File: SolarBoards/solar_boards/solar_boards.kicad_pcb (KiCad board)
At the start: 2 copper layers, 51.8 x 47 mm, 5 parts, among them J1 M55-6001242R

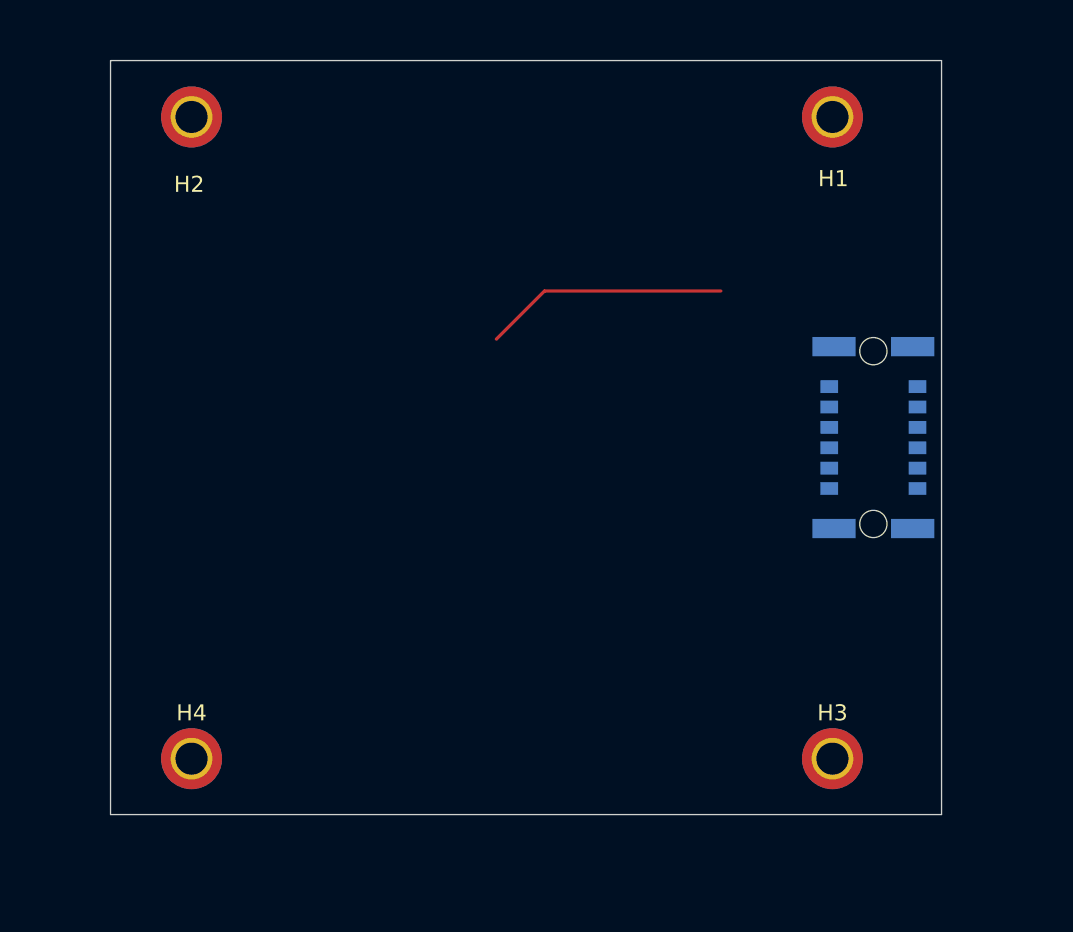
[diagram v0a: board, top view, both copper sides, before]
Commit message: Solar Board Schematic and Routing
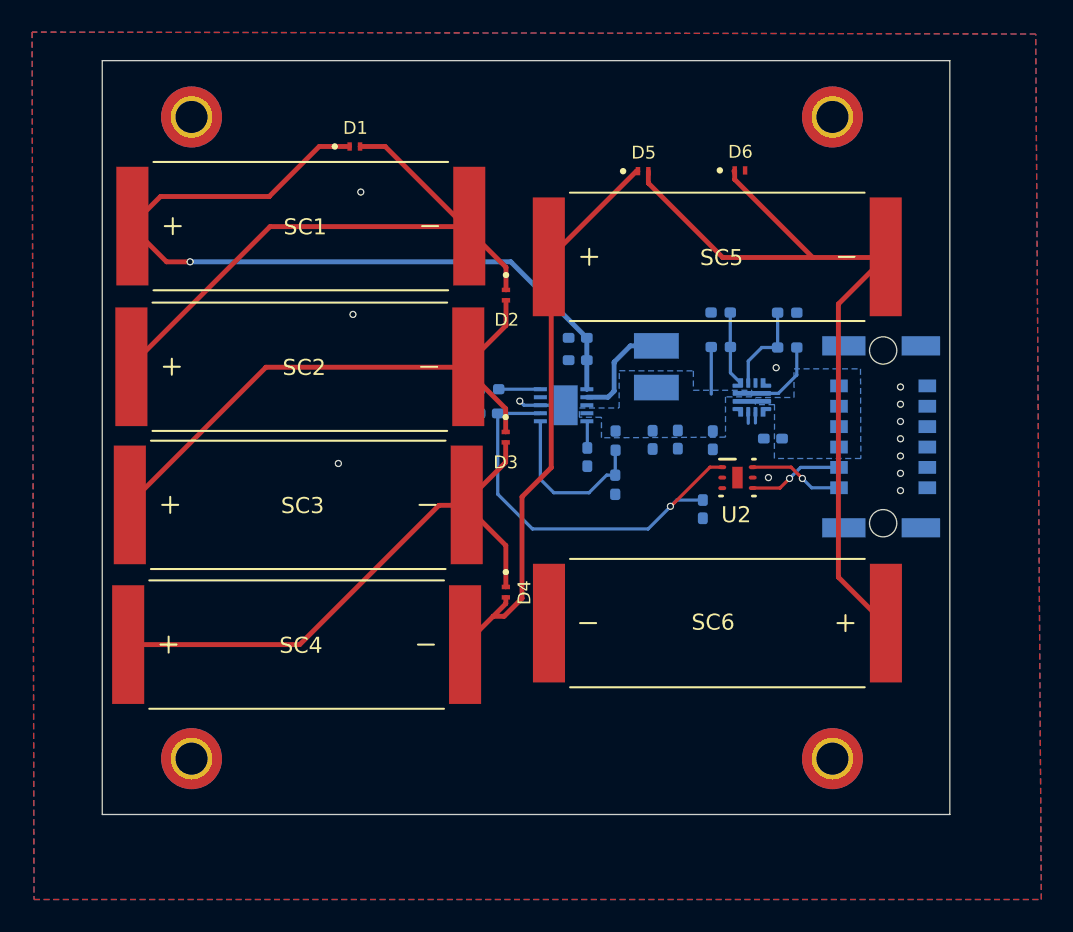
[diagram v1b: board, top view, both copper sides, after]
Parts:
- added C1: 10uF, Capacitor_SMD:C_0402_1005Metric_Pad0.74x0.62mm_HandSolder, B.Cu at (89.1, 86.4)
- added C2: 10uF, Capacitor_SMD:C_0402_1005Metric_Pad0.74x0.62mm_HandSolder, B.Cu at (89.1, 87.8)
- added C3: 10uF, Capacitor_SMD:C_0402_1005Metric_Pad0.74x0.62mm_HandSolder, B.Cu at (93.7, 92.8)
- added C4: 1uF, Capacitor_SMD:C_0402_1005Metric_Pad0.74x0.62mm_HandSolder, B.Cu at (89.7, 93.8)
- added C5: 4.7uF, Capacitor_SMD:C_0402_1005Metric_Pad0.74x0.62mm_HandSolder, B.Cu at (83.5, 91.1)
- added C6: 10uF, Capacitor_SMD:C_0402_1005Metric_Pad0.74x0.62mm_HandSolder, B.Cu at (95.3, 92.8)
- added C7: 100nF, Capacitor_SMD:C_0402_1005Metric_Pad0.74x0.62mm_HandSolder, B.Cu at (96.9, 97.1)
- added C8: 1uF, Capacitor_SMD:C_0402_1005Metric_Pad0.74x0.62mm_HandSolder, B.Cu at (97.5, 92.8)
- added C9: 1uF, Capacitor_SMD:C_0402_1005Metric_Pad0.74x0.62mm_HandSolder, B.Cu at (101.2, 92.7)
- added D1: CDBQC0130L, inspireFly:DIODFN100X60X55-2N, F.Cu at (75.2, 74.5)
- added D2: CDBQC0130L, inspireFly:DIODFN100X60X55-2N, F.Cu at (84.6, 83.8)
- added D3: CDBQC0130L, inspireFly:DIODFN100X60X55-2N, F.Cu at (84.6, 92.6)
- added D4: CDBQC0130L, inspireFly:DIODFN100X60X55-2N, F.Cu at (84.6, 102.3)
- added D5: CDBQC0130L, inspireFly:DIODFN100X60X55-2N, F.Cu at (93.2, 76.0)
- added D6: CDBQC0130L, inspireFly:DIODFN100X60X55-2N, F.Cu at (99.2, 76.0)
- added L1: 10uH, inspireFly:WE-LQFS_3818, B.Cu at (94.0, 88.2)
- added R1: 332K, Resistor_SMD:R_0402_1005Metric_Pad0.72x0.64mm_HandSolder, B.Cu at (83.5, 89.6)
- added R2: 820K, Resistor_SMD:R_0402_1005Metric_Pad0.72x0.64mm_HandSolder, B.Cu at (91.4, 92.8)
- added R3: 200K, Resistor_SMD:R_0402_1005Metric_Pad0.72x0.64mm_HandSolder, B.Cu at (91.4, 95.6)
- added R4: 549K, Resistor_SMD:R_0402_1005Metric_Pad0.72x0.64mm_HandSolder, B.Cu at (98.0, 87.0)
- added R5: 200K, Resistor_SMD:R_0402_1005Metric_Pad0.72x0.64mm_HandSolder, B.Cu at (98.0, 84.8)
- added R6: 200K, Resistor_SMD:R_0402_1005Metric_Pad0.72x0.64mm_HandSolder, B.Cu at (102.1, 84.8)
- added R7: 820K, Resistor_SMD:R_0402_1005Metric_Pad0.72x0.64mm_HandSolder, B.Cu at (102.1, 87.0)
- added SC1: Solar_Cell, inspireFly:SOLAR_KXOB25-14X1F-TR, F.Cu at (71.8, 79.5)
- added SC2: Solar_Cell, inspireFly:SOLAR_KXOB25-14X1F-TR, F.Cu at (71.8, 88.2)
- added SC3: Solar_Cell, inspireFly:SOLAR_KXOB25-14X1F-TR, F.Cu at (71.7, 96.8)
- added SC4: Solar_Cell, inspireFly:SOLAR_KXOB25-14X1F-TR, F.Cu at (71.5, 105.5)
- added SC5: Solar_Cell, inspireFly:SOLAR_KXOB25-14X1F-TR, F.Cu at (97.8, 81.4)
- added SC6: Solar_Cell, inspireFly:SOLAR_KXOB25-14X1F-TR, F.Cu at (97.8, 104.2)
- added U1: LTC3105EDD-TRPBF, inspireFly:DFN-10_DD_LIT, B.Cu at (88.2, 90.6)
- added U2: OPT3004DNPR, inspireFly:DNP0006A, F.Cu at (99.0, 95.1)
- added U3: LM73100RPWR, inspireFly:IC_LM73100RPWR, B.Cu at (99.9, 90.1)
- moved J1 0.61 mm to (108.1, 92.6), turned to -90 degrees
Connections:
- J1 pad A1: unconnected-(J1-PadA1) -> GND
- J1 pad A2: unconnected-(J1-PadA2) -> GND
- J1 pad A3: unconnected-(J1-PadA3) -> GND
- J1 pad A4: unconnected-(J1-PadA4) -> GND
- J1 pad A5: unconnected-(J1-PadA5) -> GND
- J1 pad A6: unconnected-(J1-PadA6) -> GND
- J1 pad B1: unconnected-(J1-PadB1) -> EXTERNAL_VOLTAGE
- J1 pad B2: unconnected-(J1-PadB2) -> EXTERNAL_VOLTAGE
- J1 pad B3: unconnected-(J1-PadB3) -> EXTERNAL_VOLTAGE
- J1 pad B4: unconnected-(J1-PadB4) -> EXTERNAL_VOLTAGE
- J1 pad B5: unconnected-(J1-PadB5) -> I2C_SCL
- J1 pad B6: unconnected-(J1-PadB6) -> I2C_SDA
- J1 pad SH1: unconnected-(J1-PadSH1) -> GND
- J1 pad SH2: unconnected-(J1-PadSH2) -> GND
- J1 pad SH3: unconnected-(J1-PadSH3) -> GND
- J1 pad SH4: unconnected-(J1-PadSH4) -> GND
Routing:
- net Net-(D1-K): track 0.00 -> 50.2 mm, vias 0 -> 1
- net Net-(D5-A): track 0.00 -> 50.1 mm
- net Net-(D1-A): track 0.00 -> 38.1 mm
- net Net-(D4-A): track 0.00 -> 36.0 mm
- net Net-(D3-A): track 0.00 -> 35.6 mm
- net Net-(D2-A): track 0.00 -> 34.8 mm
- net +2.2V: track 0.00 -> 26.4 mm, vias 0 -> 1
- net (no net): track 15.2 -> 0.00 mm
- net Net-(U1-FB): track 0.00 -> 10.6 mm
- net Net-(U1-VOUT): track 0.00 -> 7.93 mm
- net Net-(U1-SW): track 0.00 -> 6.72 mm
- net I2C_SDA: track 0.00 -> 5.91 mm, vias 0 -> 1
- net I2C_SCL: track 0.00 -> 5.91 mm, vias 0 -> 1
- net Net-(U3-OVLO): track 0.00 -> 5.72 mm
- net Net-(U3-EN/UVLO): track 0.00 -> 4.66 mm
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- added copper zone on B.Cu, net EXTERNAL_VOLTAGE
- added copper zone on B.Cu, net GND
- added copper zone on F.Cu, net GND
- added copper zone on B.Cu, net Net-(U1-VOUT)
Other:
- board size 51.8 x 47 mm -> 52.8 x 47 mm
